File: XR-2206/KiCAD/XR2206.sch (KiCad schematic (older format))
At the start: 15 parts, among them J1 CONN_3, J2 CONN_2, U1 XR2206

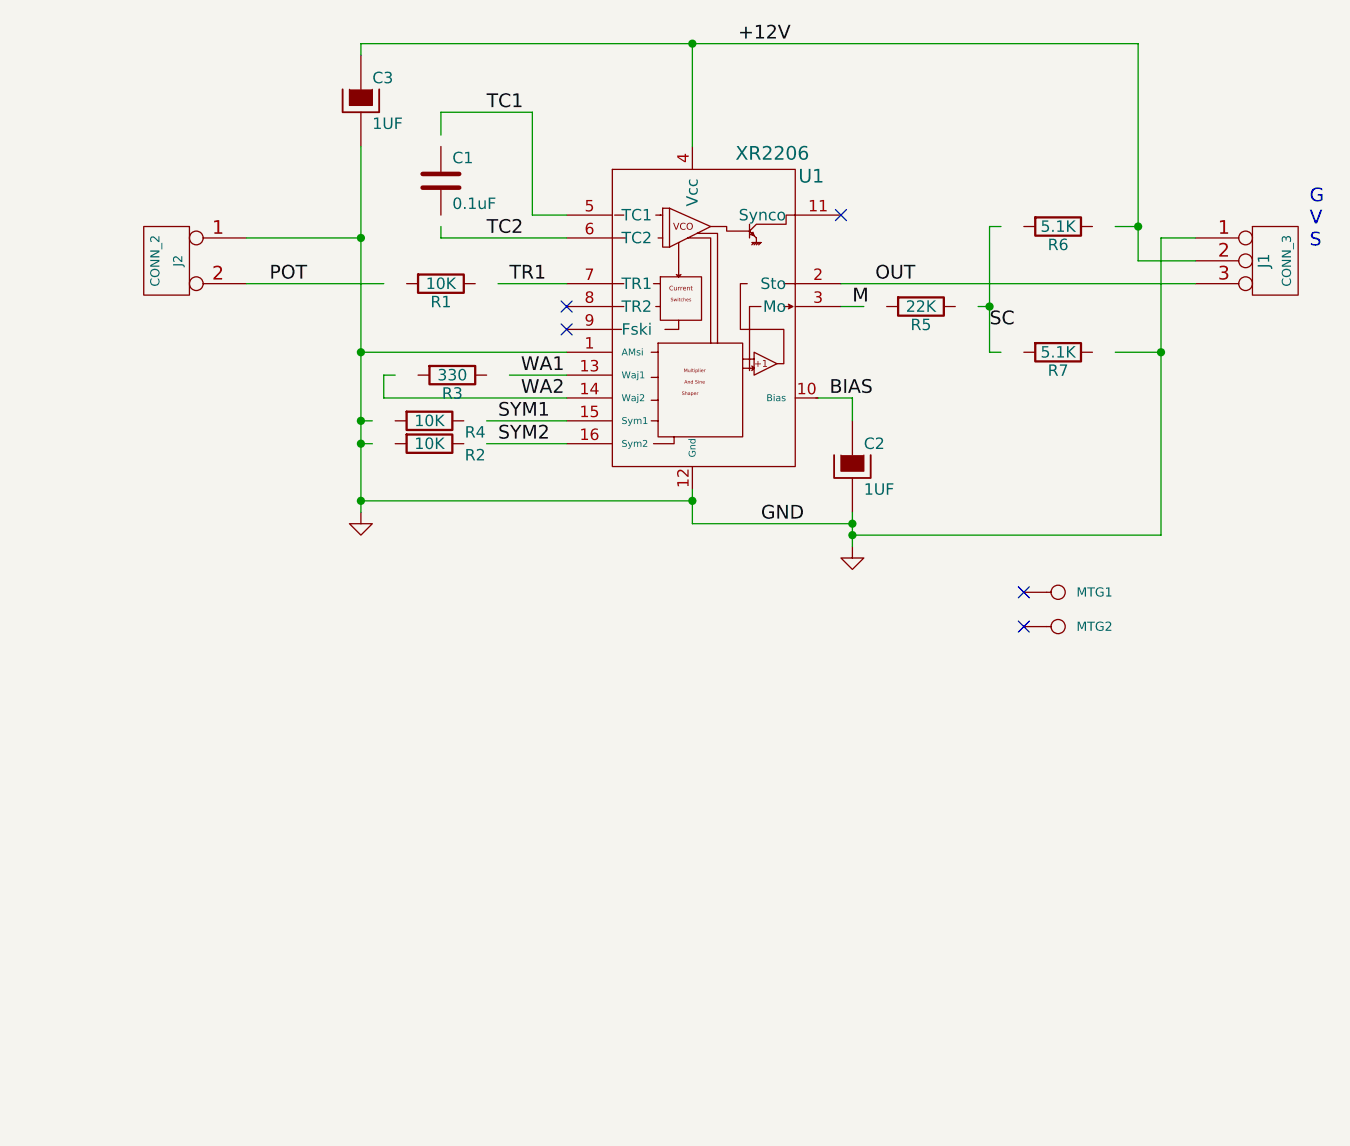
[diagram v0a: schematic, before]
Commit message: updating theremin related files
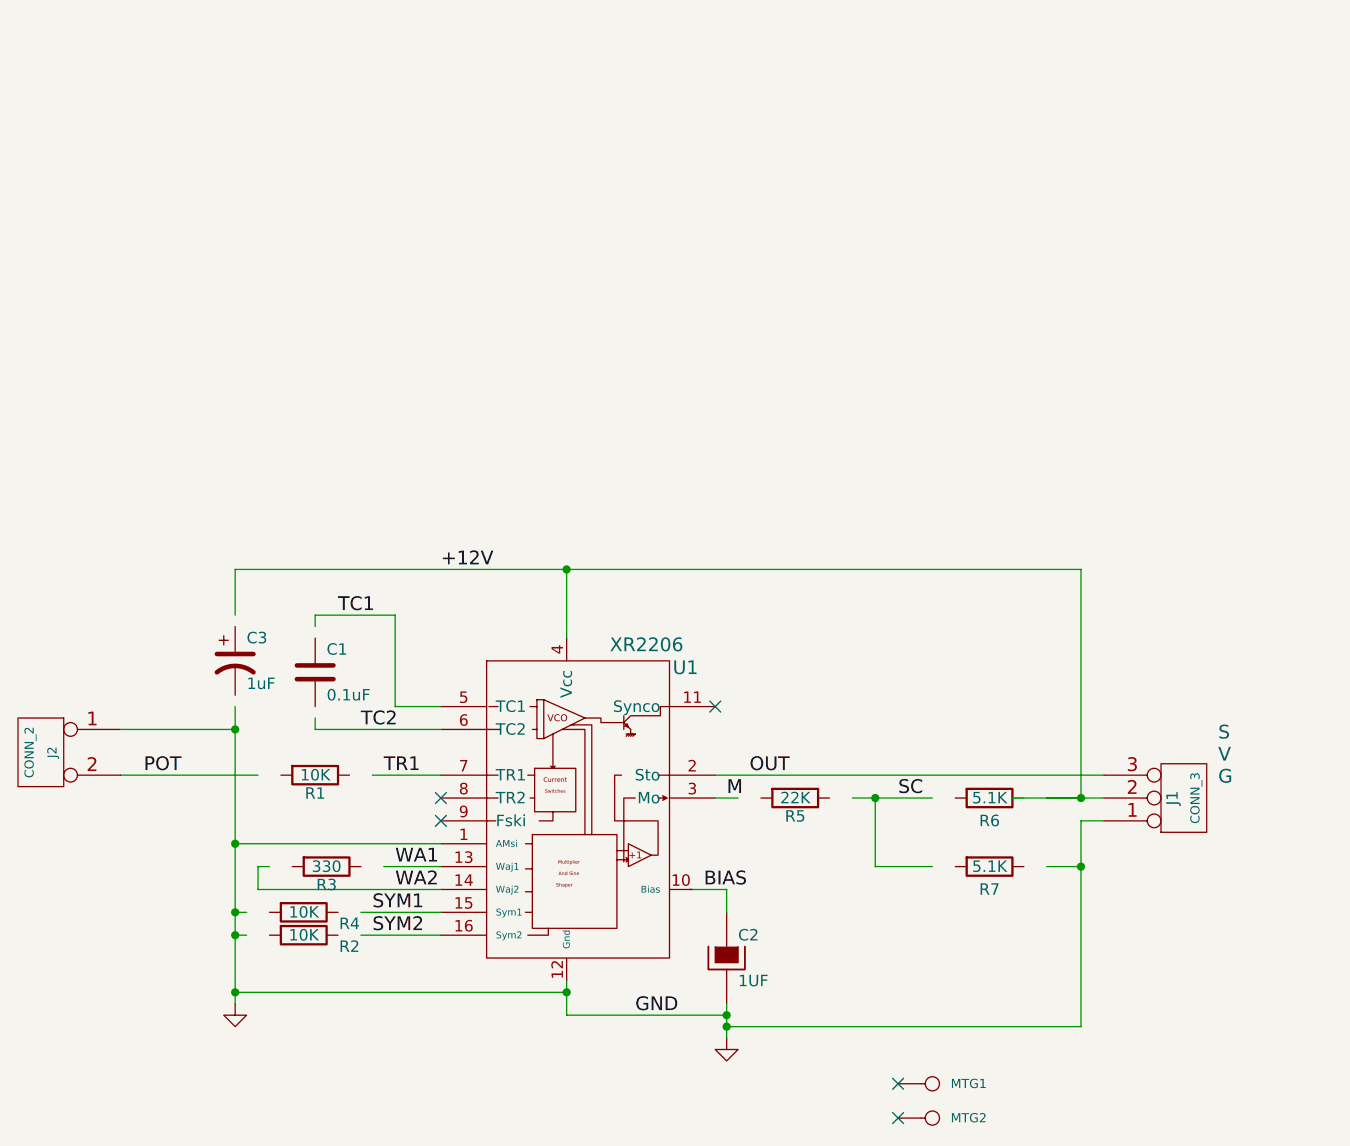
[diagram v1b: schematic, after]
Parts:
- removed C3: 1UF, symbol CAPAPOL
- added C3: 1uF, symbol CP1
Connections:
- wire segments 41 -> 52
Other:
- note added: "S\nV\nG"
- note removed: "G\nV\nS"
- moved on the sheet: C1, C2, J1, J2, MTG1, MTG2, R1, R2, R3, R4, R5, R6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
